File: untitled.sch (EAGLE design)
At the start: 11 parts

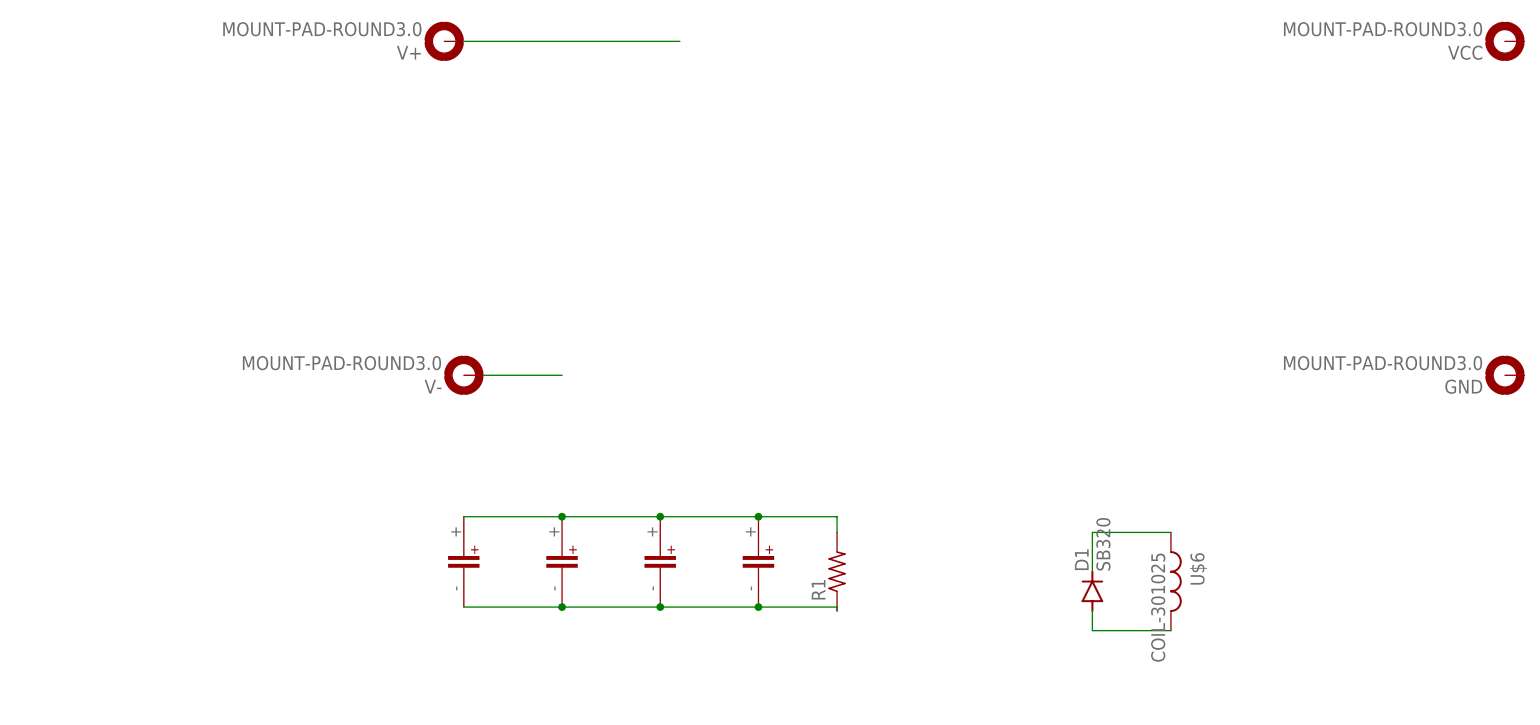
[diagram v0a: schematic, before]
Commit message: add
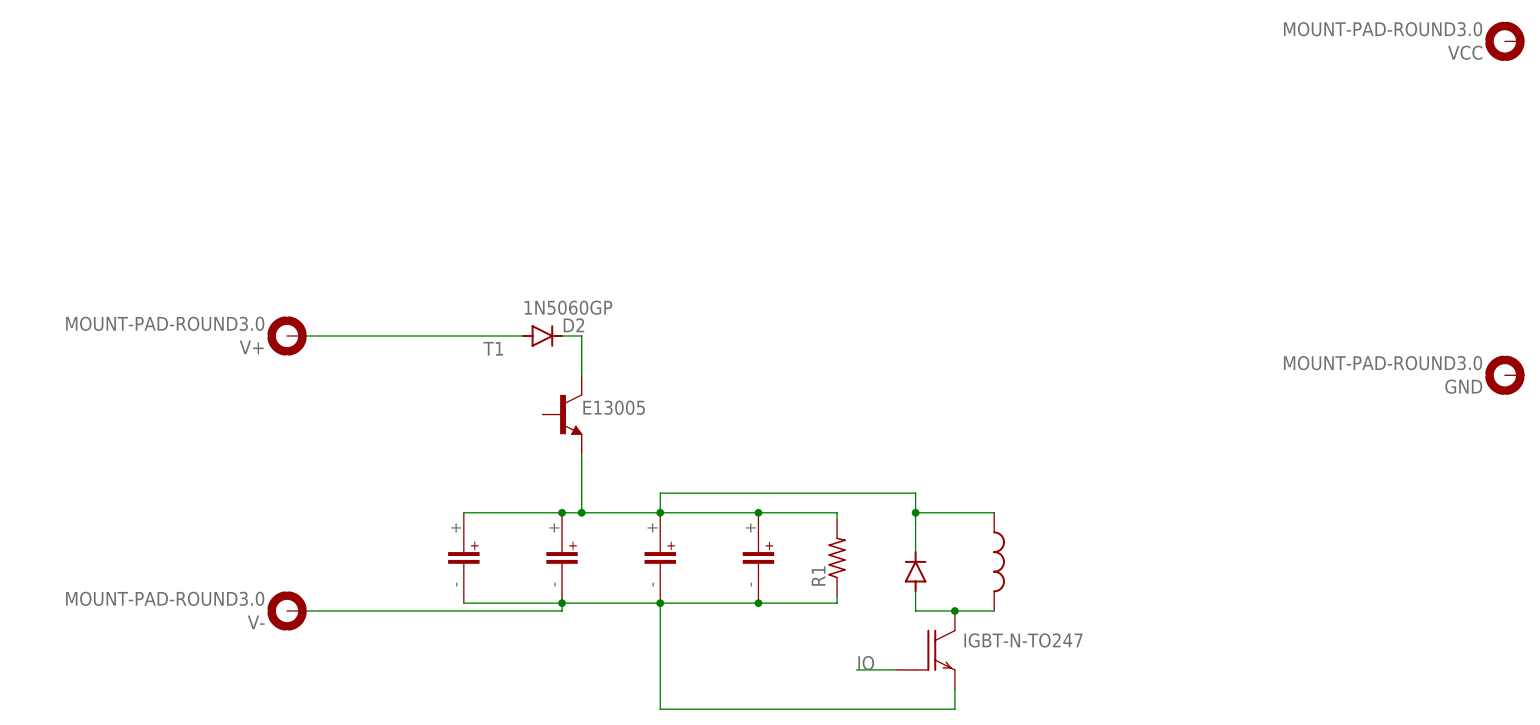
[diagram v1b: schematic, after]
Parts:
- added D2: 1N5060GP, diode:1N5060GP
- added T1: E13005, transistor:2SC1306
- added U$9: IGBT-N-TO247, untitled:IGBT-N-TO247
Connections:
- removed net N$2: R1.2, U$1.+, U$2.+, U$3.+, U$4.+
- new net IO: U$9.G
- net GND: now also R1.1, U$1.-, U$2.-, U$3.-, U$4.-, U$9.E
- net N$1: now also D2.C, T1.C; no longer R1.1, U$1.-, U$2.-, U$3.-, U$4.-
- net N$3: now also R1.2, T1.E, U$1.+, U$2.+, U$3.+, U$4.+
- net N$4: now also U$9.C
- net N$8: now also D2.A
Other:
- moved on the sheet: R1, V+, V-
